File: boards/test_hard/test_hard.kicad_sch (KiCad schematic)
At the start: 19 parts, among them J4 GND, J5 3V3, J6 5V, J7 Conn_01x04, J8 Conn_01x02, U2 ESP32-S3-MINI-1, U3 SN65HVD230

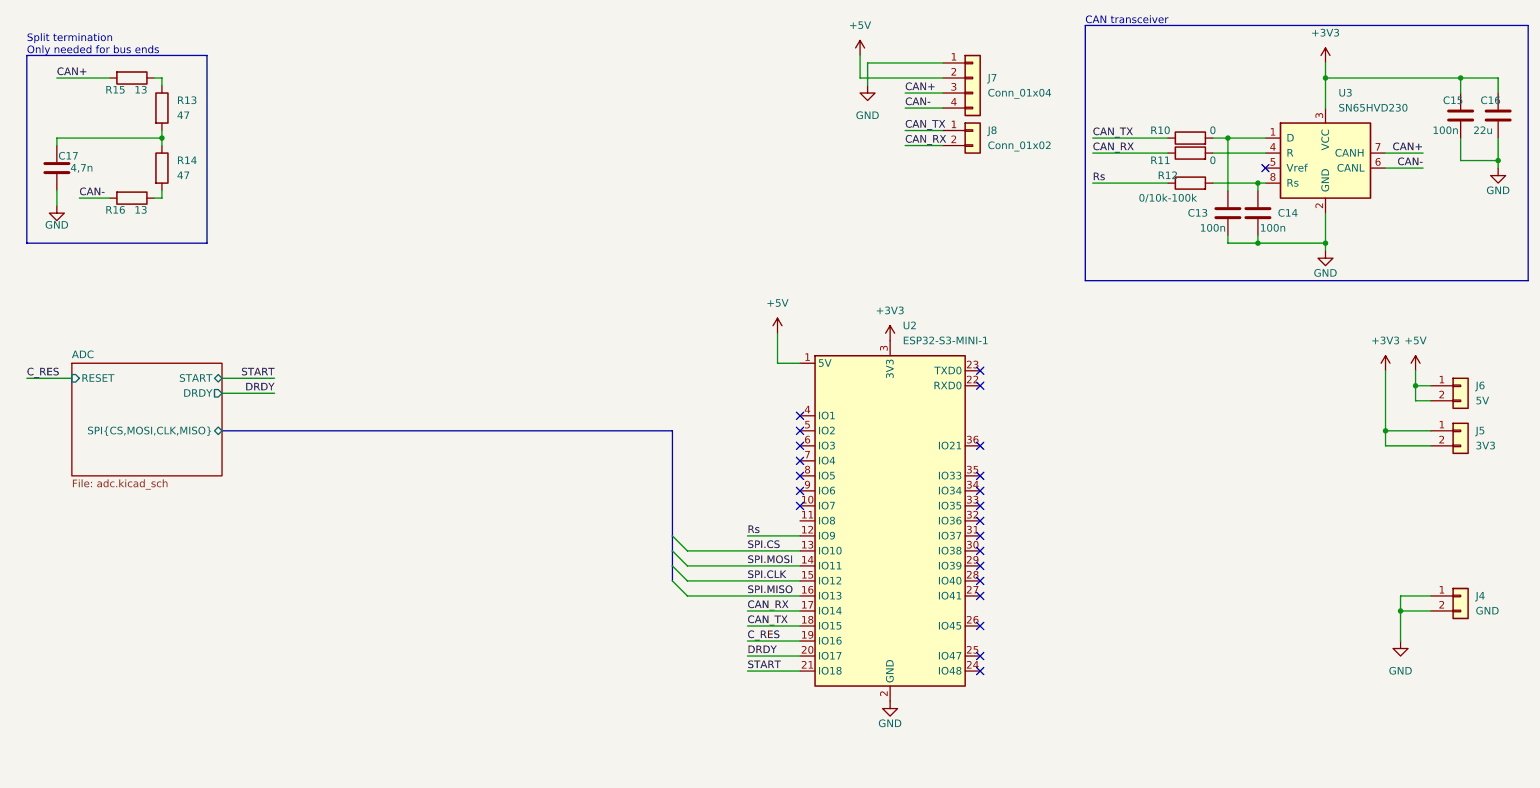
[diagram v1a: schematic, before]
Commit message: Aktueller Stand
Signed-off-by: Philipp Macher <philipp-macher@web.de>
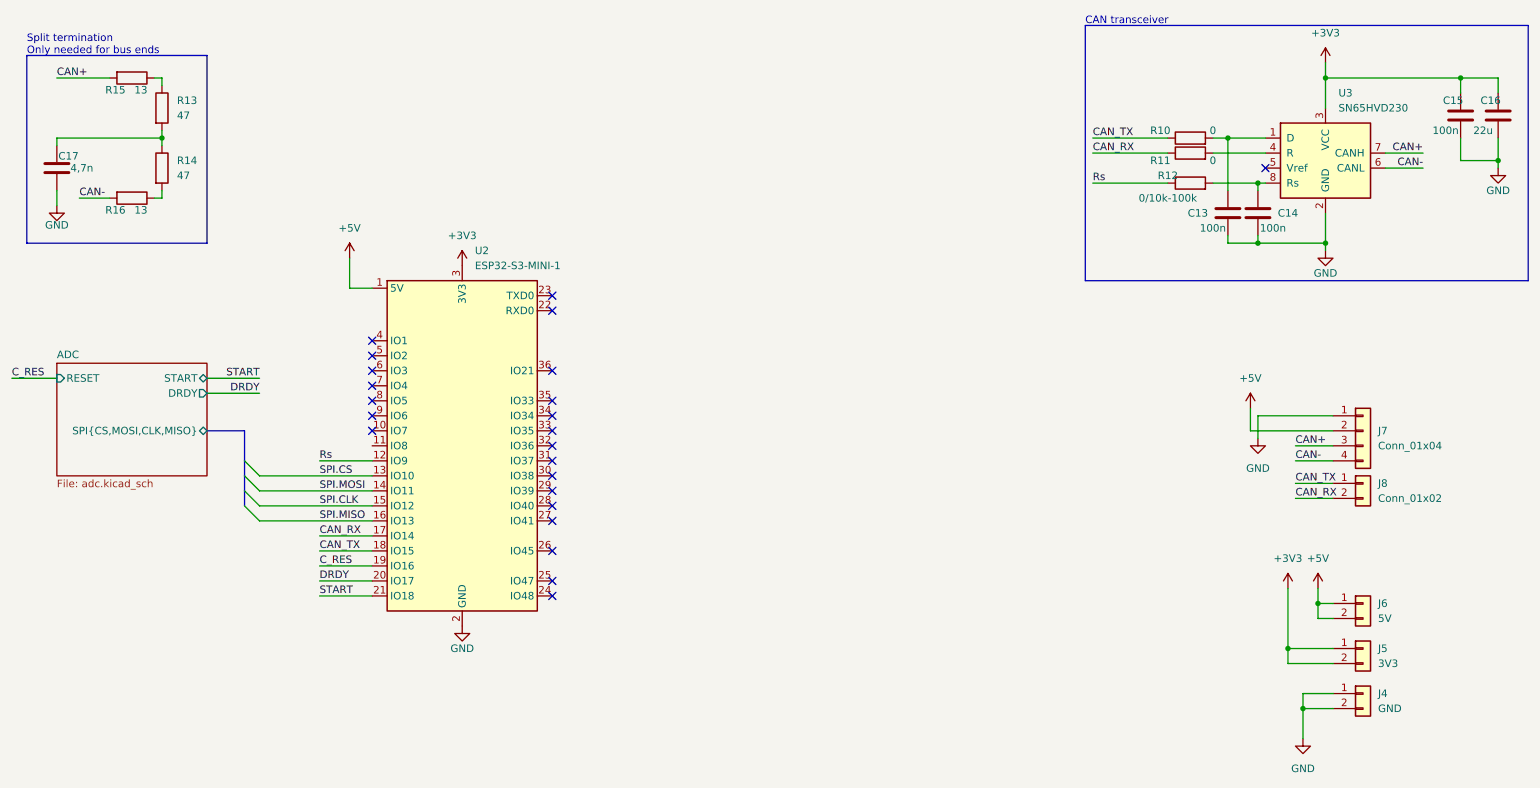
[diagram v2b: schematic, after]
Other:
- moved on the sheet: J4, J5, J6, J7, J8, U2
